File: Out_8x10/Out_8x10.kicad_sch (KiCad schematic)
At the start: 68 parts, among them J1 Conn_01x06, J2 nmount SW Debug, J3 USB_C_Receptacle_USB2.0, J4 Conn_01x06, SW1 Reset, SW2 Boot, SW3 ADDRESS, U1 ADM3483, U2 W25Q128JVSIQ, U3 RP2040, U4 SN74AHCT1G125, U5 AP2112K-3.3, Y1 12MHz,18pF

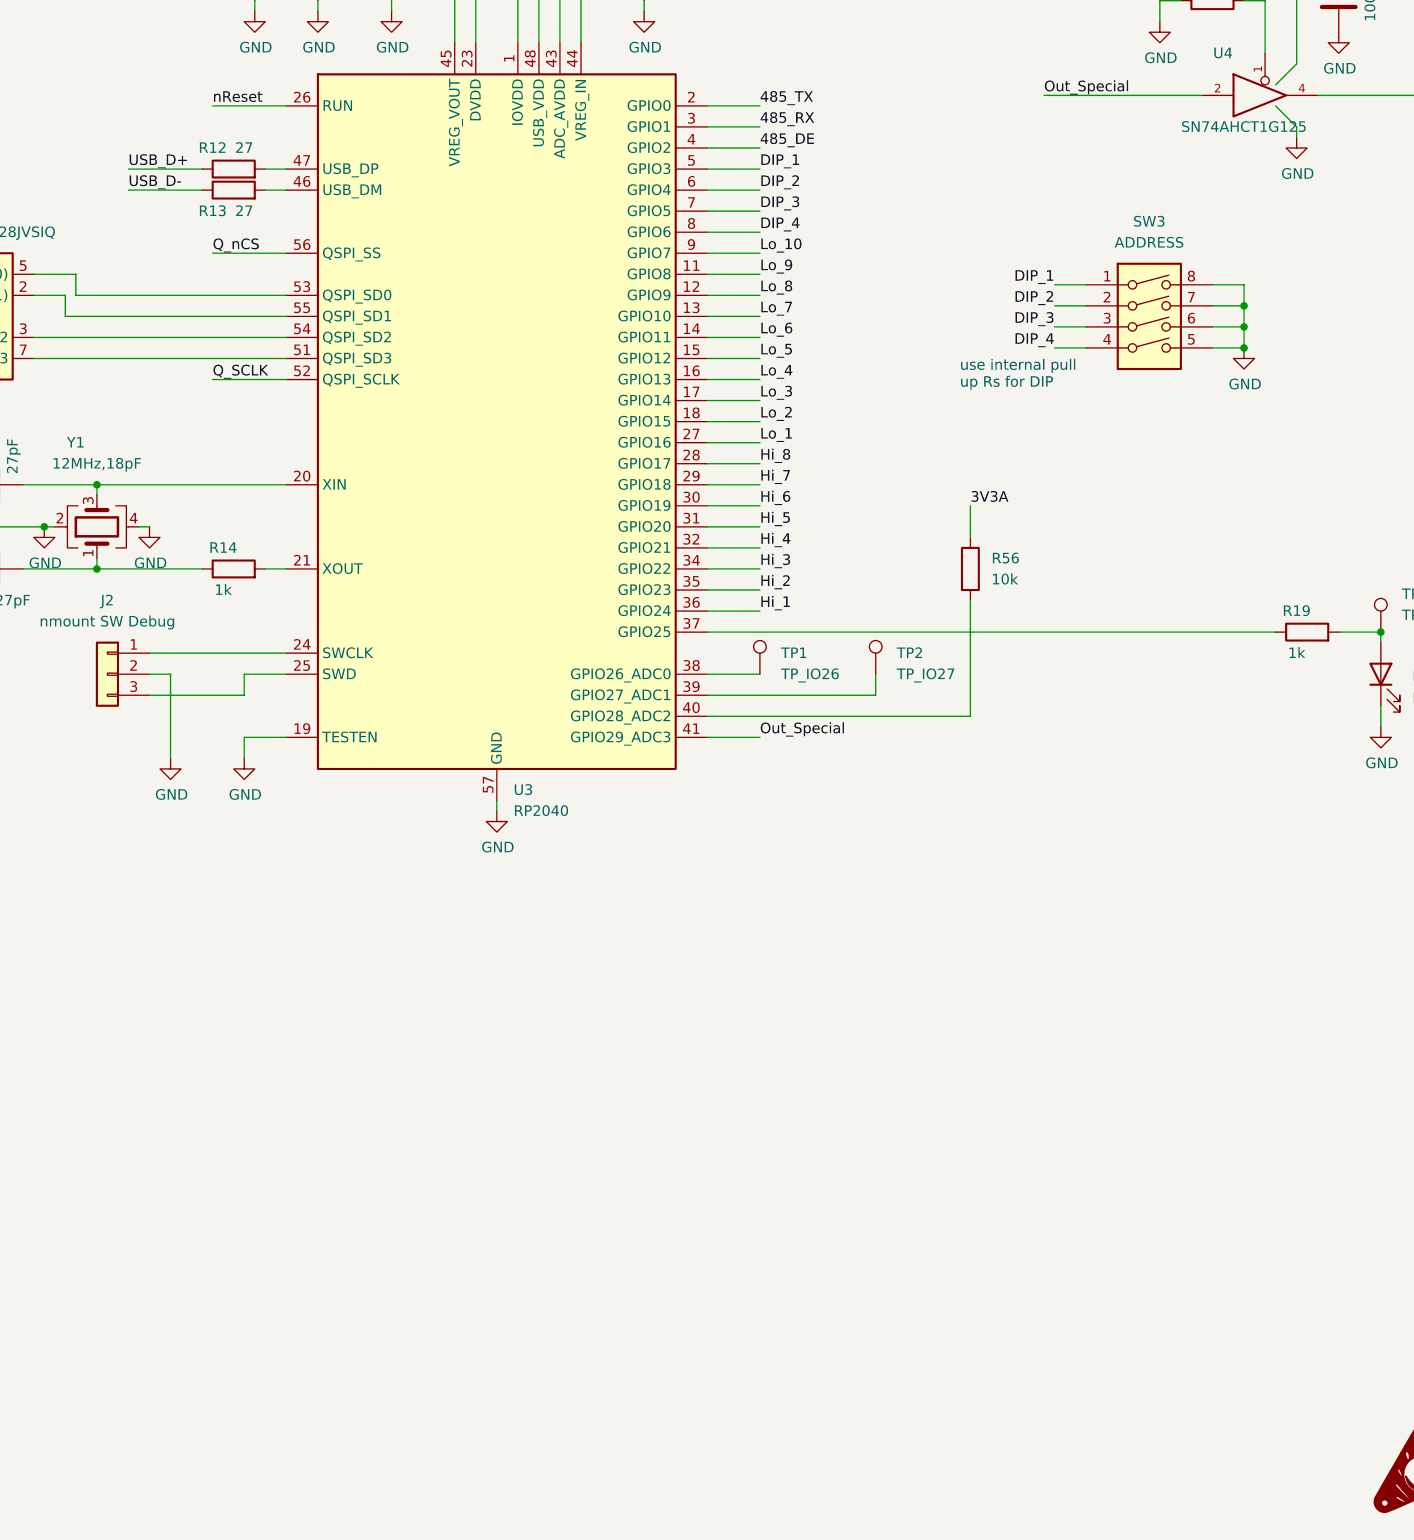
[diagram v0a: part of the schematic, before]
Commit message: Analog DIP
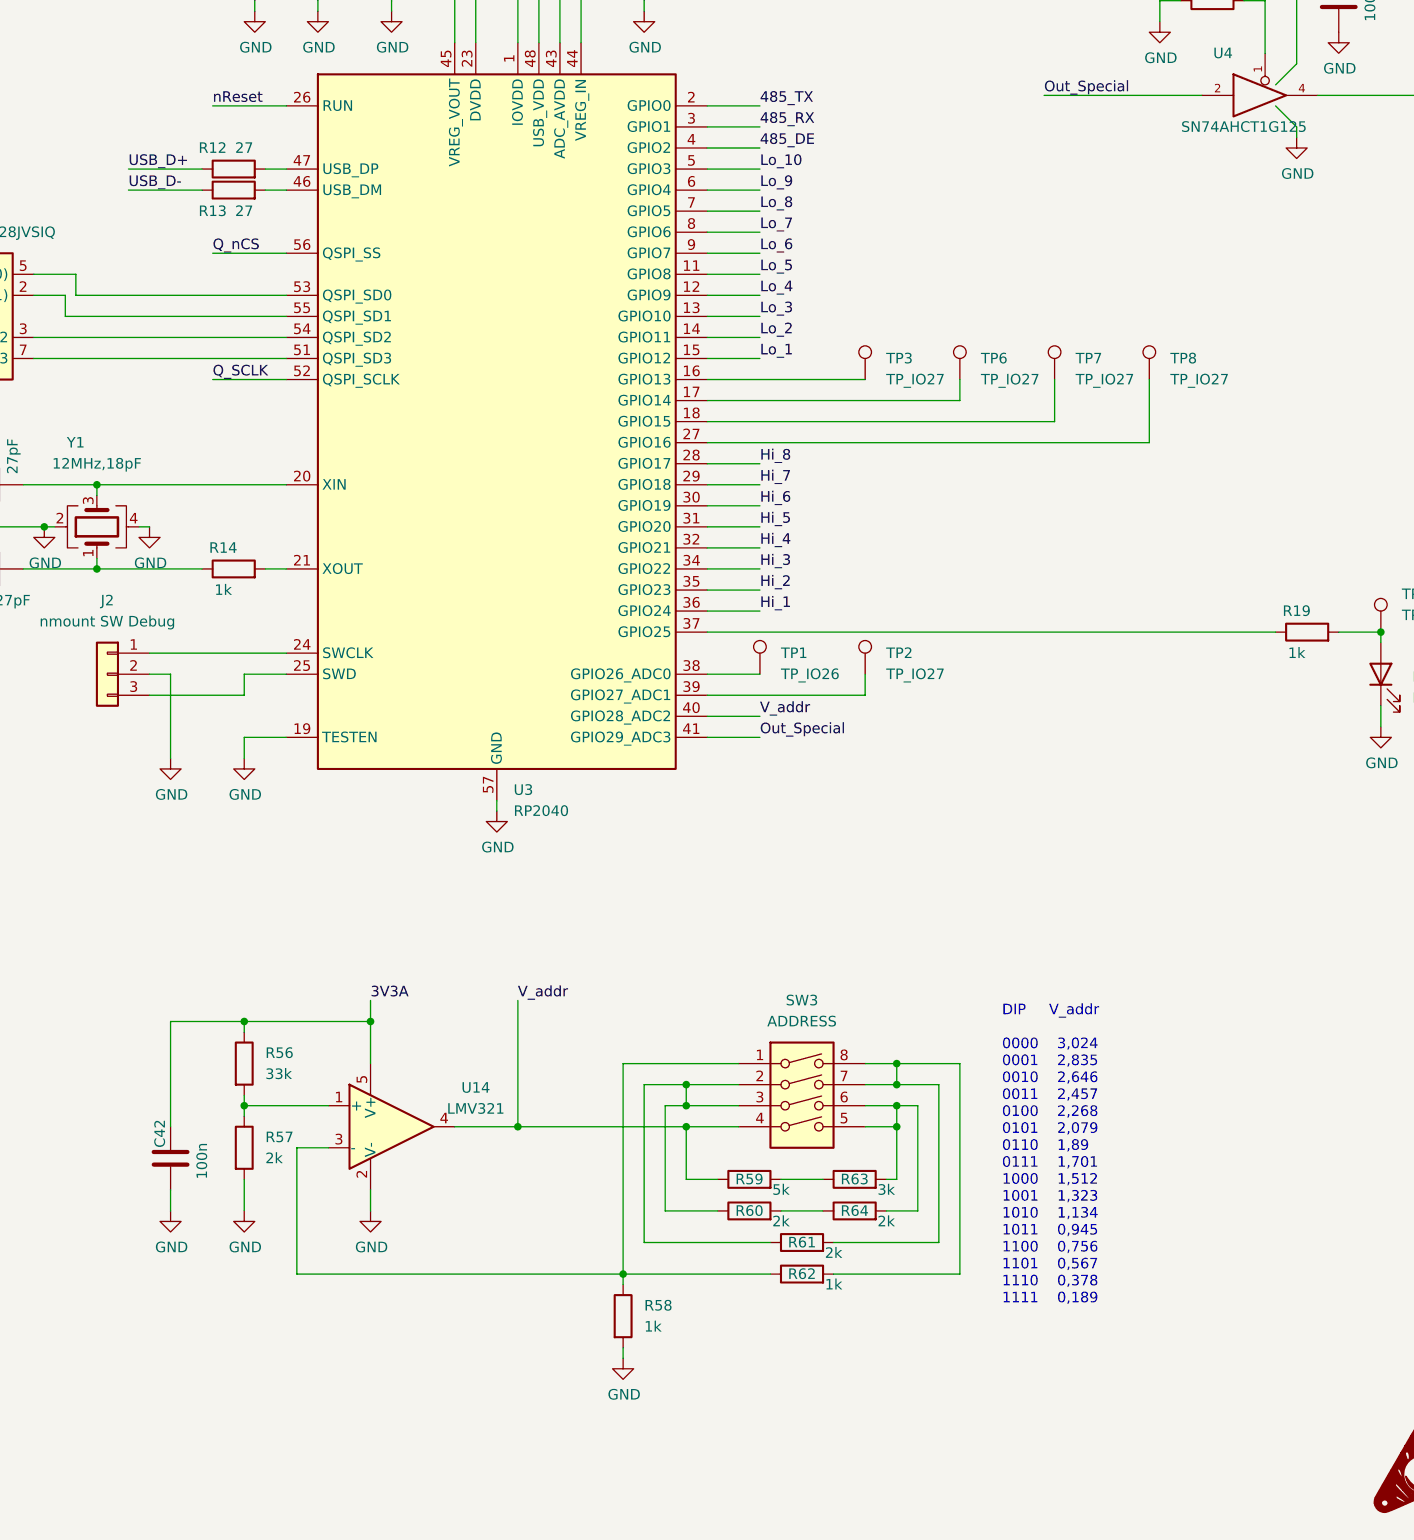
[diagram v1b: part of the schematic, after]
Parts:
- added C42: 100n, Capacitor_SMD:C_0402_1005Metric, symbol Device:C
- added R57, R60, R61, R64: 2k, Resistor_SMD:R_0603_1608Metric, symbol Device:R
- added R58, R62: 1k, Resistor_SMD:R_0402_1005Metric, symbol Device:R
- added R59: 5k, Resistor_SMD:R_0603_1608Metric, symbol Device:R
- added R63: 3k, Resistor_SMD:R_0603_1608Metric, symbol Device:R
- added TP3, TP6, TP7, TP8: TP_IO27, TestPoint:TestPoint_Pad_D1.0mm, symbol Connector:TestPoint
- added U14: LMV321, Package_TO_SOT_SMD:SOT-23-5, symbol Amplifier_Operational:LMV321
- R56: value 10k -> 33k
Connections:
- net 3V3A: now also C42.1, U14.5 (V+)
- net GND: now also C42.2, R57.2, R58.2, U14.2 (V-); no longer SW3.5, SW3.6, SW3.7, SW3.8
- net Lo_1: now also U3.15 (GPIO12); no longer U3.27 (GPIO16)
- net Lo_10: now also U3.5 (GPIO3); no longer U3.9 (GPIO7)
- net Lo_2: now also U3.14 (GPIO11); no longer U3.18 (GPIO15)
- net Lo_3: now also U3.13 (GPIO10); no longer U3.17 (GPIO14)
- net Lo_4: now also U3.12 (GPIO9); no longer U3.16 (GPIO13)
- net Lo_5: now also U3.11 (GPIO8); no longer U3.15 (GPIO12)
- net Lo_6: now also U3.9 (GPIO7); no longer U3.14 (GPIO11)
- net Lo_7: now also U3.8 (GPIO6); no longer U3.13 (GPIO10)
- net Lo_8: now also U3.7 (GPIO5); no longer U3.12 (GPIO9)
- net Lo_9: now also U3.6 (GPIO4); no longer U3.11 (GPIO8)
- net at R56.2: now also R57.1, U14.1 (+); no longer U3.40 (GPIO28_ADC2)
- net DIP_1: no longer names the net of SW3.1
- net DIP_1: now also R58.1, R62.1, U14.3 (-); no longer U3.5 (GPIO3)
- net DIP_2: no longer names the net of SW3.2
- net DIP_2: now also SW3.3, R60.1, R61.1; no longer U3.6 (GPIO4)
- removed net DIP_3: SW3.3, U3.7 (GPIO5)
- net DIP_4 renamed V_addr
- net V_addr: now also U3.40 (GPIO28_ADC2), R59.1, U14.4; no longer U3.8 (GPIO6)
- new net: R61.2, R62.2, SW3.7, SW3.8
- new net: TP6.1, U3.17 (GPIO14)
- new net: TP3.1, U3.16 (GPIO13)
- new net: TP7.1, U3.18 (GPIO15)
- new net: TP8.1, U3.27 (GPIO16)
- new net: R59.2, R63.1
- new net: R63.2, R64.2, SW3.5, SW3.6
- new net: R60.2, R64.1
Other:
- note added: "DIP V_addr 0000 3,024 0001 2,835 0010 2,646 0011 2,457 0100 2,268 0101 2,079 0110 1,89 0111 1,701 1000 1,512 1001 1,323 1010 1,134 1011 0,945 1100 0,756 1101 0,567 1110 0,378 1111 0,189"
- note removed: "use internal pull up Rs for DIP"
- moved on the sheet: TP2
